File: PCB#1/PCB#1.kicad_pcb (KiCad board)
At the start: 2 copper layers, 48 parts, among them J2 Conn_01x02, P1 USB_C_Plug_USB2.0, Q1 BSS138, U1 RP2040, U2 ICM-20948, U3 NCP1117-3.3_SOT223, U4 W25Q128JVS, U5 NCP1117-1.8_SOT223, U7 MPL115A1, U8 TCA9406DC, Y1 Crystal_GND24

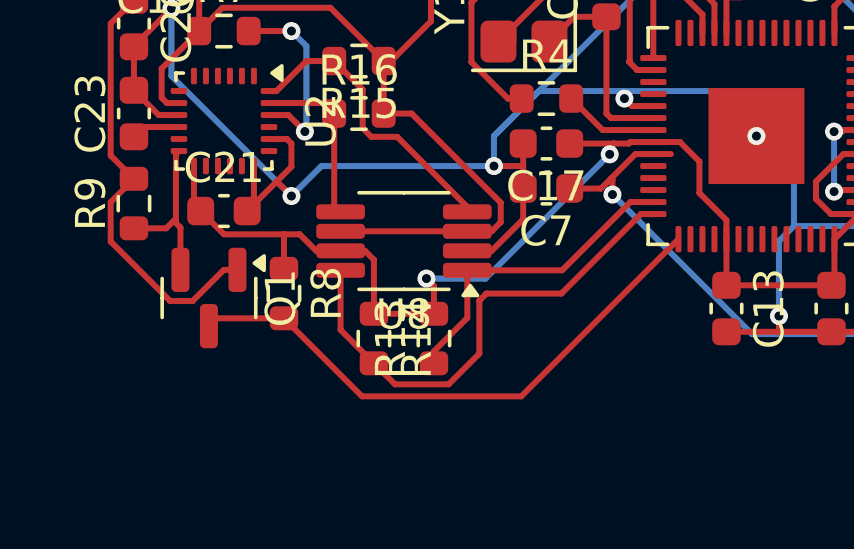
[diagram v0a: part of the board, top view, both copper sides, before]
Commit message: Add files via upload
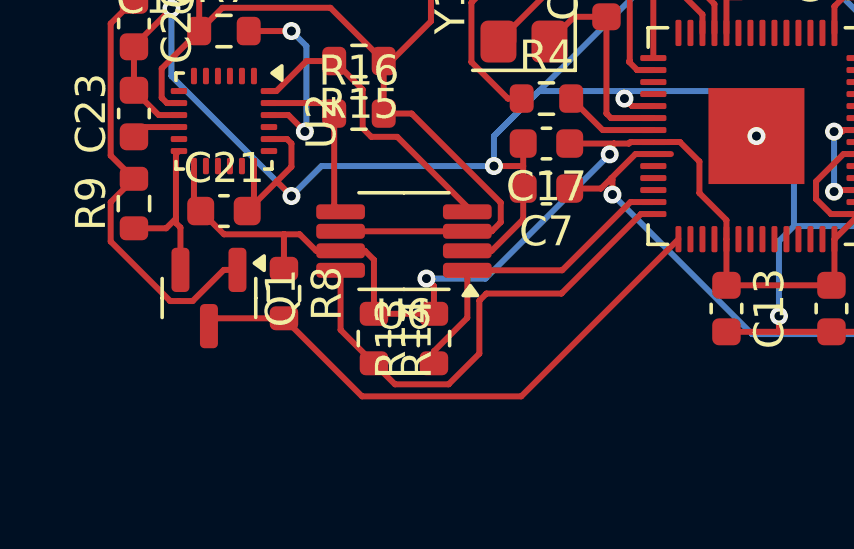
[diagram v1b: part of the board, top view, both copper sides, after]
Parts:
- Q1: value BSS138 -> onsemi BSS138
- U1: value RP2040 -> Raspberry Pi RP2040
- U2: value ICM-20948 -> TDK InvenSense ICM-20948
- U3: value NCP1117-3.3_SOT223 -> onsemi NCP1117DT33G
- U5: value NCP1117-1.8_SOT223 -> onsemi NCP1117DT33G
- U6: renamed from U8; value TCA9406DC -> TI TCA9406DCTR
- U7: value MPL115A1 -> NXP MPL115A1T1
- Y1: value Crystal_GND24 -> ABRACON ABM8-272-T3
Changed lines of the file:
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@@
 			)
 		)
-		(property "Value" "ICM-20948"
+		(property "Value" "TDK InvenSense ICM-20948"
 			(at 0 3.25 90)
 			(layer "F.Fab")
@@
 			)
 		)
-		(property "Value" "Crystal_GND24"
+		(property "Value" "ABRACON ABM8-272-T3"
 			(at 0 2.45 90)
 			(layer "F.Fab")
@@
 			)
 		)
-		(property "Value" "NCP1117-3.3_SOT223"
+		(property "Value" "onsemi NCP1117DT33G"
 			(at 0 4.5 90)
 			(layer "F.Fab")
@@
 			)
 		)
-		(property "Value" "MPL115A1"
+		(property "Value" "NXP MPL115A1T1"
 			(at 0 3.45 0)
 			(layer "F.Fab")
@@
 			)
 		)
-		(property "Value" "NCP1117-1.8_SOT223"
+		(property "Value" "onsemi NCP1117DT33G"
 			(at 0 4.5 0)
 			(layer "F.Fab")
@@
 			)
 		)
-		(property "Value" "RP2040"
+		(property "Value" "Raspberry Pi RP2040"
 			(at 0 4.83 90)
 			(layer "F.Fab")
@@
 			)
 		)
-		(property "Value" "BSS138"
+		(property "Value" "onsemi BSS138"
 			(at 0 2.4 90)
 			(layer "F.Fab")
@@
 		(descr "VSSOP, 8 Pin (https://www.jedec.org/standards-documents/docs/mo-187-f), generated with kicad-footprint-generator ipc_gullwing_generator.py")
 		(tags "VSSOP SO JEDEC-MO-187-AA Texas_DGK0008A")
-		(property "Reference" "U8"
+		(property "Reference" "U6"
 			(at 0 -2.45 0)
 			(layer "F.SilkS")
@@
 			)
 		)
-		(property "Value" "TCA9406DC"
+		(property "Value" "TI TCA9406DCTR"
 			(at 0 2.45 0)
 			(layer "F.Fab")
